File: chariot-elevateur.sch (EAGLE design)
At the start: 63 parts, among them P1 RG500, Q1 DMN2056U, Q2 DMN2056U, U1 WIZ820IO

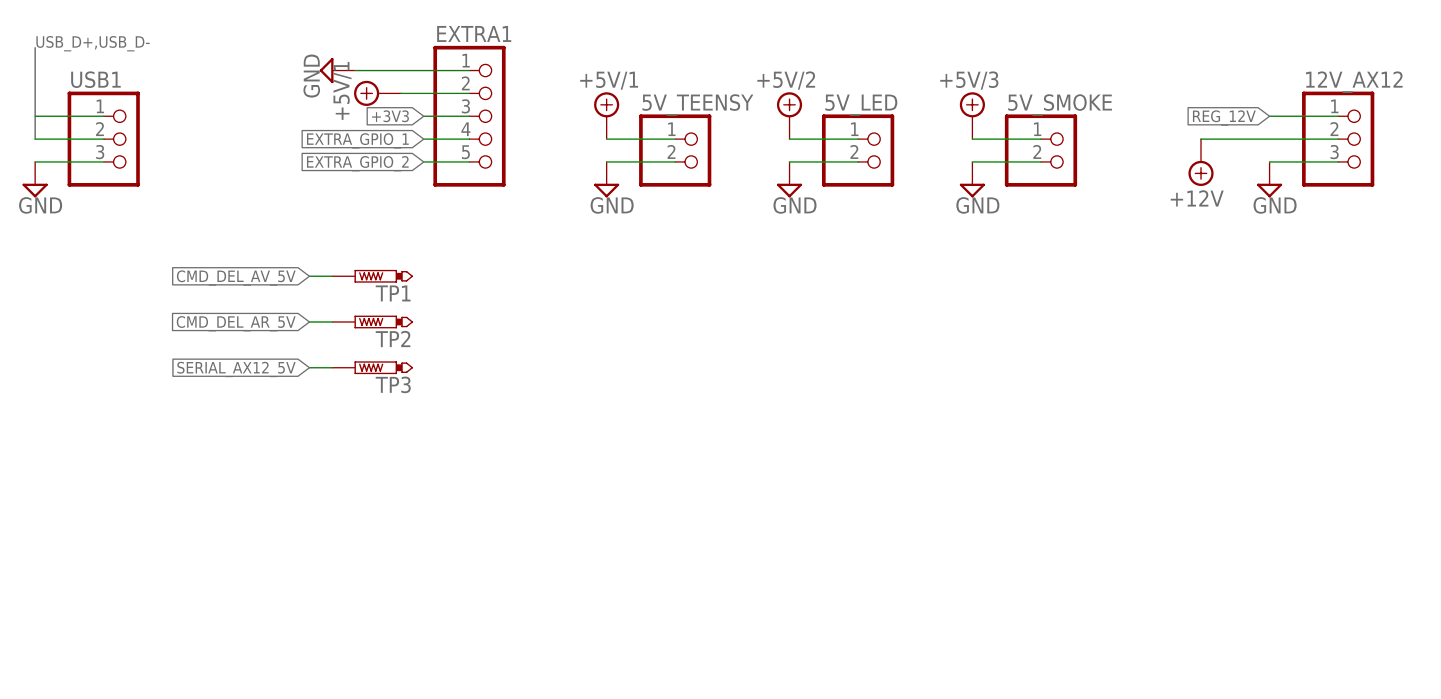
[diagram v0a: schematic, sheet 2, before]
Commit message: all done, missing doc
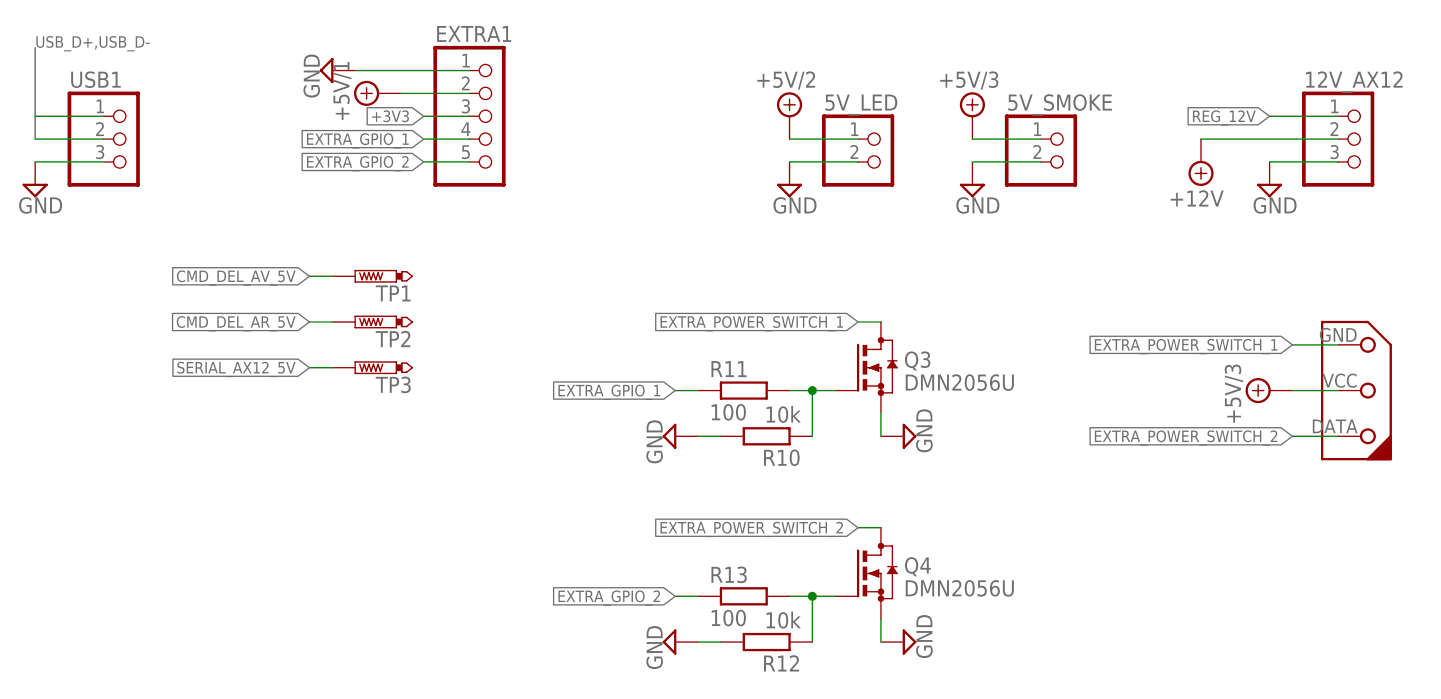
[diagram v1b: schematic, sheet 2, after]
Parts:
- removed 5V_TEENSY: (no value), pinhead:PINHD-1X2
- added FUMIGENE1: DYNAMIXEL-1X03XL, 1NTech_pinhead:DYNAMIXEL-1X03XL
- added Q3, Q4: DMN2056U, transistor-small-signal:BSS123
- added R10, R12: 10k, resistor:R-EU_R0805
- added R11, R13: 100, resistor:R-EU_R0805
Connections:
- new net EXTRA_POWER_SWITCH_1: FUMIGENE1.GND, Q3.D
- new net EXTRA_POWER_SWITCH_2: FUMIGENE1.DATA, Q4.D
- new net N$12: Q4.G, R12.1, R13.2
- new net N$9: Q3.G, R10.1, R11.2
- net +5V/1: no longer 5V_TEENSY.1
- net +5V/3: now also FUMIGENE1.DYN_VCC
- net EXTRA_GPIO_1: now also R11.1
- net EXTRA_GPIO_2: now also R13.1
- net GND: now also Q3.S, Q4.S, R10.2, R12.2; no longer 5V_TEENSY.2

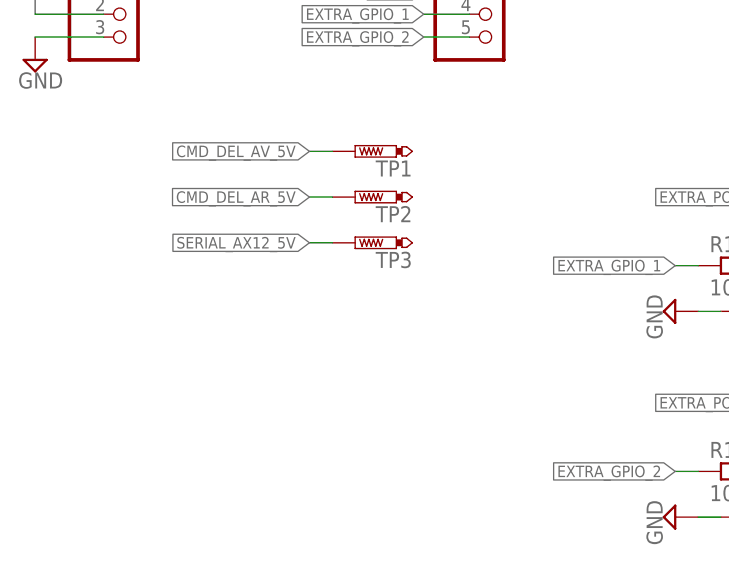
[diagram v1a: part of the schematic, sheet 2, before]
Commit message: CAM files are ready
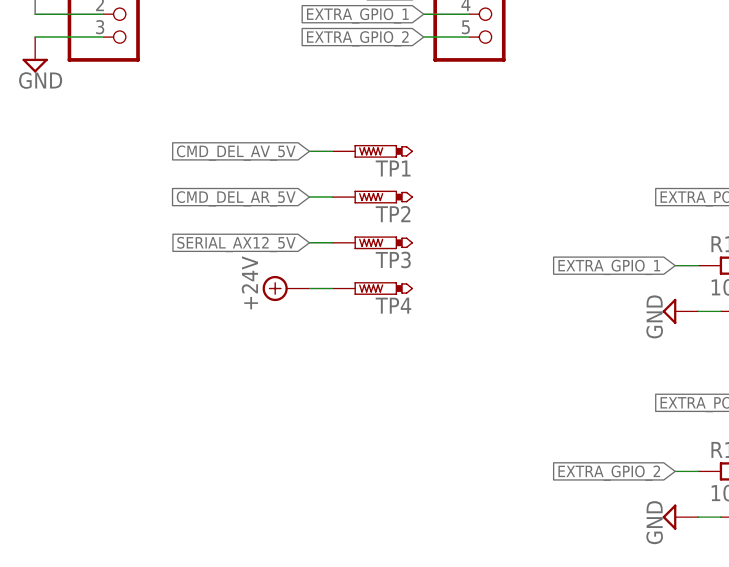
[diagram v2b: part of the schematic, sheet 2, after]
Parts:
- added TP4: PTR1PAD1-13, testpad:PTR1PAD1-13
- renumbered FUMIGENE1 to EXTRA
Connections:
- net +24V: now also TP4.TP
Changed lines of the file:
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@@
 <part name="R11" library="resistor" library_urn="urn:adsk.eagle:library:348" deviceset="R-EU_" device="R0805" package3d_urn="urn:adsk.eagle:package:23553/2" value="100"/>
 <part name="SUPPLY69" library="supply2" library_urn="urn:adsk.eagle:library:372" deviceset="GND" device=""/>
-<part name="FUMIGENE1" library="1NTech_pinhead" deviceset="DYNAMIXEL-1X03" device="XL">
+<part name="EXTRA" library="1NTech_pinhead" deviceset="DYNAMIXEL-1X03" device="XL">
 <attribute name="RS" value="688-3283"/>
 </part>
@@
 <part name="R13" library="resistor" library_urn="urn:adsk.eagle:library:348" deviceset="R-EU_" device="R0805" package3d_urn="urn:adsk.eagle:package:23553/2" value="100"/>
 <part name="SUPPLY72" library="supply2" library_urn="urn:adsk.eagle:library:372" deviceset="GND" device=""/>
+<part name="TP4" library="testpad" library_urn="urn:adsk.eagle:library:385" deviceset="PTR1" device="PAD1-13" package3d_urn="urn:adsk.eagle:package:27946/1"/>
+<part name="SUPPLY54" library="supply2" library_urn="urn:adsk.eagle:library:372" deviceset="+24V" device=""/>
 </parts>
 <sheets>
@@
 <attribute name="VALUE" x="88.265" y="65.405" size="1.778" layer="96" rot="R270"/>
 </instance>
-<instance part="FUMIGENE1" gate="G$1" x="165.1" y="68.58" smashed="yes" rot="R90">
+<instance part="EXTRA" gate="G$1" x="165.1" y="68.58" smashed="yes" rot="R90">
 <attribute name="RS" x="165.1" y="68.58" size="1.778" layer="96" rot="R90" display="off"/>
 </instance>
@@
 <attribute name="VALUE" x="88.265" y="42.545" size="1.778" layer="96" rot="R270"/>
 </instance>
+<instance part="TP4" gate="G$1" x="55.88" y="66.04" smashed="yes" rot="R90">
+<attribute name="NAME" x="62.23" y="65.024" size="1.778" layer="95" rot="R180"/>
+<attribute name="TP_SIGNAL_NAME" x="58.42" y="67.31" size="1.778" layer="97" rot="R90"/>
+</instance>
+<instance part="SUPPLY54" gate="+24V" x="48.26" y="66.04" smashed="yes" rot="R90">
+<attribute name="VALUE" x="45.085" y="63.5" size="1.778" layer="96" rot="R90"/>
+</instance>
 </instances>
 <busses>
@@
 </segment>
 <segment>
-<pinref part="FUMIGENE1" gate="G$1" pin="DYN_VCC"/>
+<pinref part="EXTRA" gate="G$1" pin="DYN_VCC"/>
 <pinref part="SUPPLY70" gate="G$1" pin="+5V/3"/>
 <wire x1="160.02" y1="68.58" x2="165.1" y2="68.58" width="0.1524" layer="91"/>
@@
 </segment>
 <segment>
-<pinref part="FUMIGENE1" gate="G$1" pin="GND"/>
+<pinref part="EXTRA" gate="G$1" pin="GND"/>
 <wire x1="165.1" y1="73.66" x2="160.02" y2="73.66" width="0.1524" layer="91"/>
 <label x="160.02" y="73.66" size="1.27" layer="95" rot="R180" xref="yes"/>
@@
 <net name="EXTRA_POWER_SWITCH_2" class="2">
 <segment>
-<pinref part="FUMIGENE1" gate="G$1" pin="DATA"/>
+<pinref part="EXTRA" gate="G$1" pin="DATA"/>
 <wire x1="165.1" y1="63.5" x2="160.02" y2="63.5" width="0.1524" layer="91"/>
 <label x="160.02" y="63.5" size="1.27" layer="95" rot="R180" xref="yes"/>
@@
 </segment>
 </net>
+<net name="+24V" class="3">
+<segment>
+<pinref part="TP4" gate="G$1" pin="TP"/>
+<wire x1="53.34" y1="66.04" x2="50.8" y2="66.04" width="0.1524" layer="91"/>
+<pinref part="SUPPLY54" gate="+24V" pin="+24V"/>
+</segment>
+</net>
